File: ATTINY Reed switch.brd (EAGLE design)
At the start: 22.6 x 39.5 mm, 8 parts

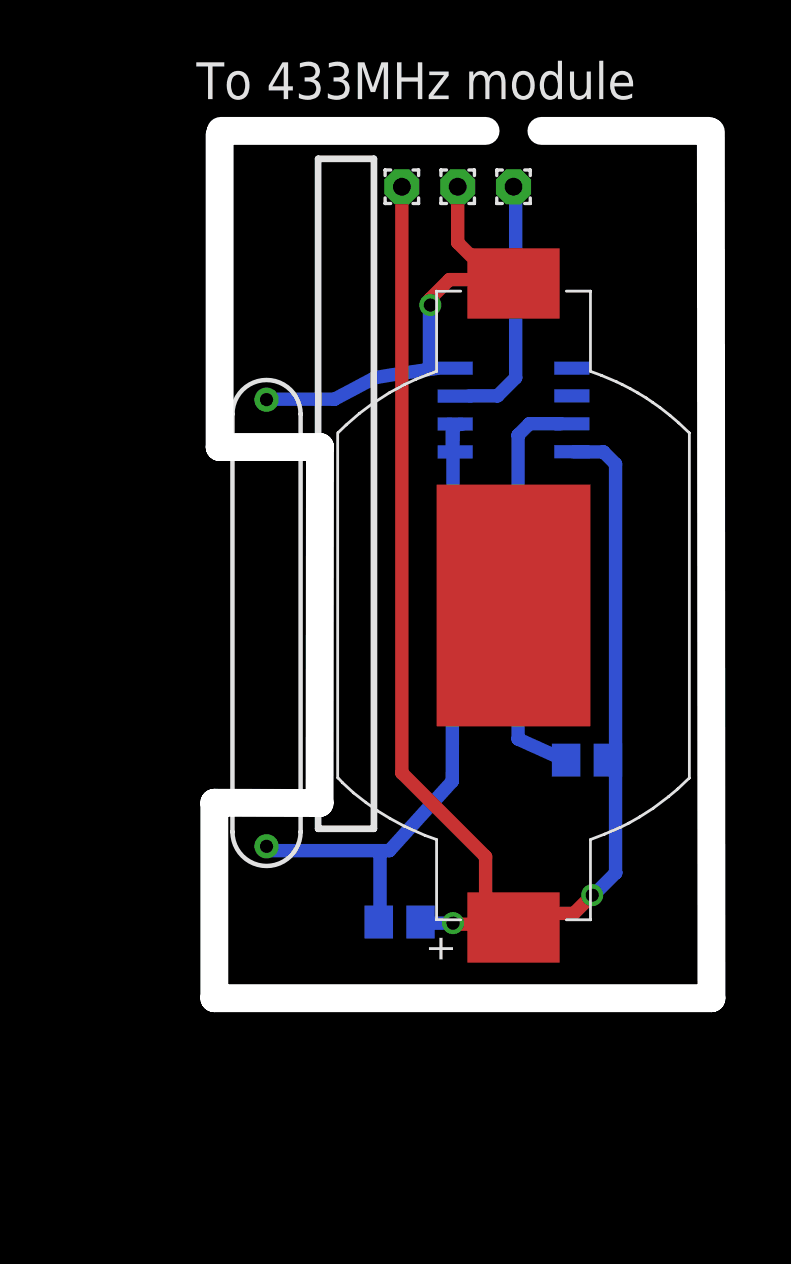
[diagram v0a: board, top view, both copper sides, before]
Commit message: Add files via upload
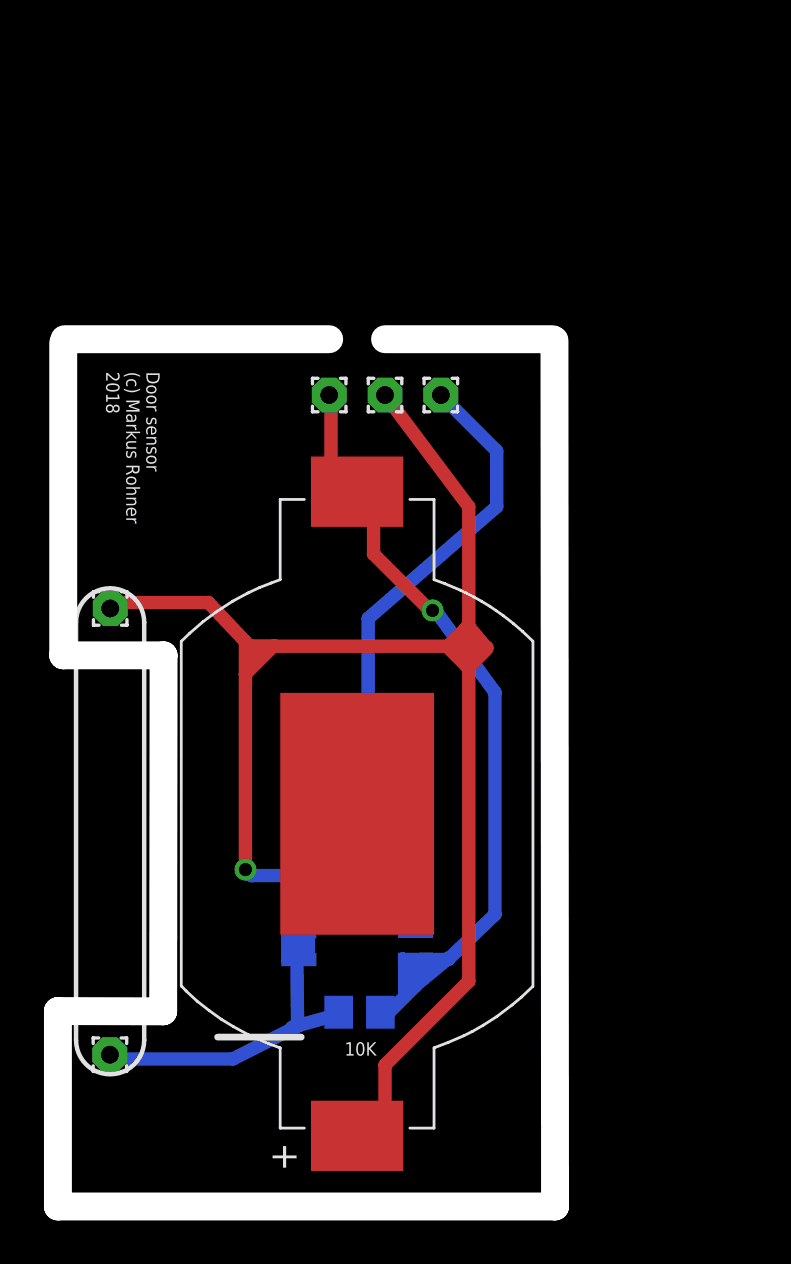
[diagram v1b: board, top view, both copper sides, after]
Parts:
- added E$6: (no value), wirepad:1,6/0,8
- E$5: device eagle-ltspice:R0805 -> wirepad:1,6/0,8
- moved E$9 43.5 mm to (3.23, 7.50)
- moved E$1 24.2 mm to (14.5, 13.7)
- moved E$5 17.9 mm to (18.3, 37.5), flipped to the top
- moved E$2 11.9 mm to (14.5, 18.5)
- moved E$3 11.9 mm to (3.24, 17.7)
- moved E$7 10.0 mm to (13.2, 37.5)
- moved E$8 10.0 mm to (15.7, 37.5)
- moved E$4 4.49 mm to (14.6, 9.43)
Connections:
- removed net S$11: E$8.1
- removed net S$13: E$7.1
- new net S$14: E$5.1
- new net VCC: E$8.1
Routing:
- net VCC: track 6.84 -> 68.2 mm, vias 0 -> 1
- net S$13: track 34.6 -> 1.55 mm
- net S$14: track 0.00 -> 26.3 mm
- net S$10: track 18.3 -> 1.23 mm
- net S$4: track 26.4 -> 13.5 mm
- net S$12: track 11.3 -> 2.08 mm
- net S$9: track 8.01 -> 0.01 mm
- net S$22: track 0.00 -> 5.00 mm
- net S$21: track 0.00 -> 4.92 mm
- net S$11: track 4.34 -> 0.00 mm, vias 0 -> 1
- net S$7: track 0.00 -> 3.51 mm, vias 1 -> 0
- net GND: track 29.2 -> 30.8 mm
- net S$5: track 0.00 -> 1.30 mm, vias 1 -> 0
- net S$3: track 3.52 -> 2.24 mm
- net S$2: track 0.00 -> 1.19 mm, vias 1 -> 0
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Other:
- board text added: "10K"
- board text added: "Door sensor (c) Markus Rohner 2018"
- board text removed: "To 433MHz module"
